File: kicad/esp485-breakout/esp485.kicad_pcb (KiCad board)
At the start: 2 copper layers, 25.4 x 26.2 mm, 15 parts, among them J1 Conn_01x08, J2 Conn_01x08, U1 MAX3485, U2 ESP-WROOM-02

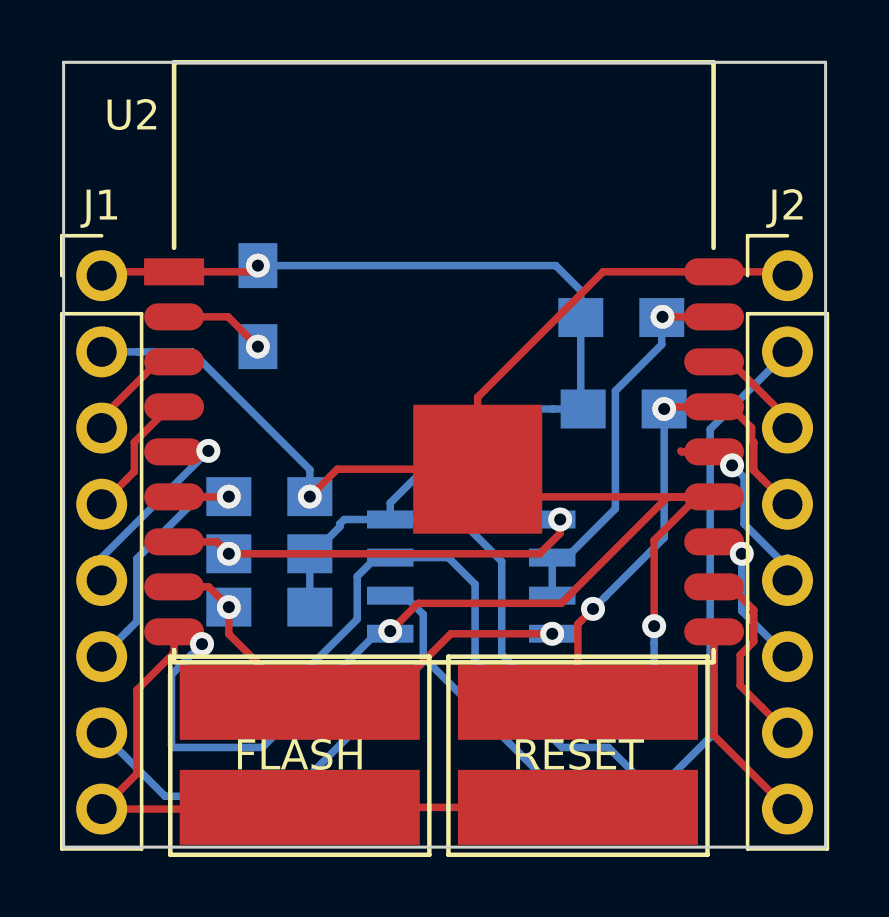
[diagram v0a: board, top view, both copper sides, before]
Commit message: all done probably
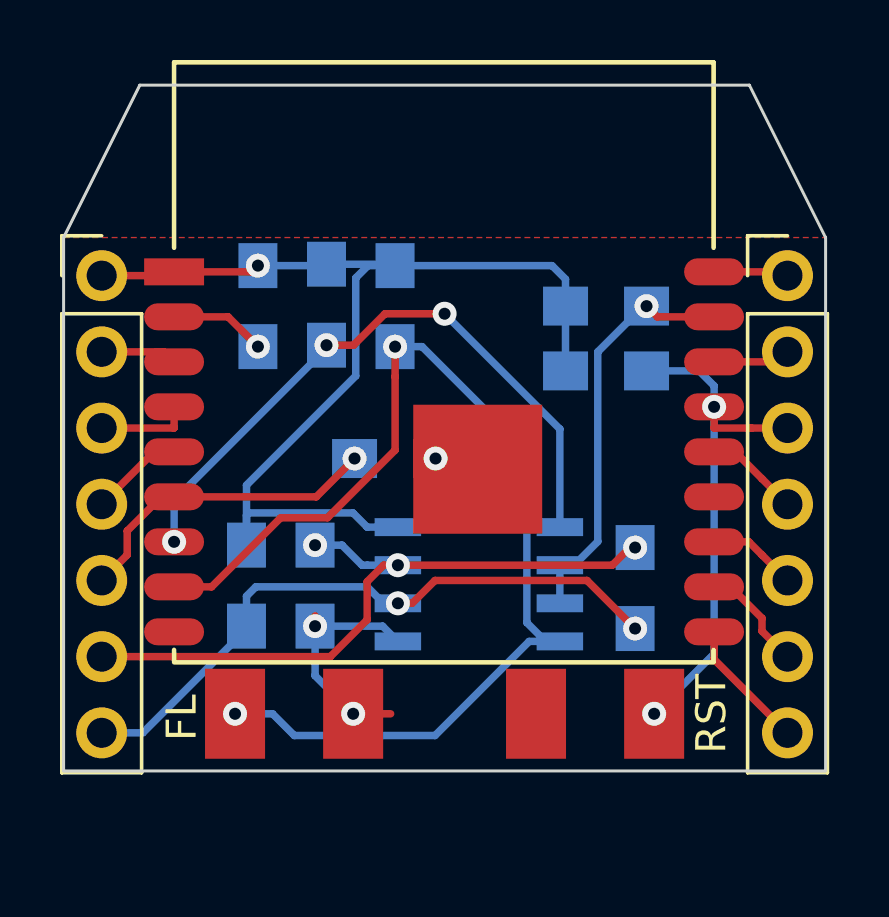
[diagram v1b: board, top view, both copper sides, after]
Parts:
- removed FLASH, RESET: SW_Push, tact:generic tactile switch
- added FL: SW_Push, tact:tactile_switch_smd_4x3mm_2p, F.Cu at (136.0, 111.1)
- added RST: SW_Push, tact:tactile_switch_smd_4x3mm_2p, F.Cu at (145.9, 111.1)
- J1, J2: value Conn_01x08 -> Conn_01x07; footprint Pin_Headers:Pin_Header_Straight_1x08_Pitch2.54mm -> Pin_Headers:Pin_Header_Straight_1x07_Pitch2.54mm
- moved R10 15.5 mm to (147.3, 106.9)
- moved R4 12.8 mm to (134.4, 106.9)
- moved R5 12.6 mm to (136.7, 106.9), turned to 270 degrees
- moved R3 10.9 mm to (139.3, 97.5), turned to 90 degrees
- moved R2 8.52 mm to (137.0, 97.5), turned to 90 degrees
- moved R9 4.38 mm to (139.3, 102.6)
- moved R7 1.40 mm to (146.4, 99.7)
- moved R8 0.64 mm to (146.4, 97.5)
- moved U1 0.36 mm to (142.1, 106.8)
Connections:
- J1 pad 2: GND -> Net-(J1-Pad2)
- R10 pad 1: Net-(J2-Pad2) -> Net-(J1-Pad6)
- R5 pad 1: Net-(J2-Pad2) -> Net-(J1-Pad6)
- R7 pad 2: Net-(J2-Pad4) -> Net-(J2-Pad3)
- R9 pad 1: Net-(J1-Pad6) -> Net-(J1-Pad5)
- U1 pad 7: Net-(J2-Pad2) -> Net-(J1-Pad6)
- U2 pad 10: Net-(J2-Pad8) -> Net-(J2-Pad7)
- U2 pad 11: Net-(J2-Pad7) -> Net-(J2-Pad6)
- U2 pad 12: Net-(J2-Pad6) -> Net-(J2-Pad5)
- U2 pad 14: Net-(J2-Pad5) -> Net-(J2-Pad4)
- U2 pad 15: Net-(J2-Pad4) -> Net-(J2-Pad3)
- U2 pad 16: Net-(J2-Pad3) -> Net-(J2-Pad2)
- U2 pad 3: Net-(J1-Pad3) -> Net-(J1-Pad2)
- U2 pad 4: Net-(J1-Pad4) -> Net-(J1-Pad3)
- U2 pad 5: Net-(J1-Pad5) -> Net-(J1-Pad4)
- U2 pad 6: Net-(J1-Pad6) -> Net-(J1-Pad5)
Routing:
- net GND: track 97.7 -> 11.0 mm, vias 4 -> 3
- net Net-(J2-Pad2): track 39.5 -> 2.58 mm
- net Net-(R3-Pad1): track 15.7 -> 38.0 mm
- net Net-(J2-Pad4): track 17.2 -> 3.17 mm, vias 2 -> 0
- net Net-(J2-Pad3): track 3.54 -> 17.4 mm, vias 0 -> 2
- net Net-(J1-Pad6): track 10.5 -> 23.1 mm, vias 1 -> 3
- net Net-(R2-Pad1): track 13.8 -> 21.6 mm, vias 2 -> 3
- net +3V3: track 44.9 -> 37.1 mm
- net Net-(J2-Pad8): track 6.92 -> 0.00 mm
- net Net-(J2-Pad5): track 7.27 -> 2.98 mm, vias 1 -> 0
- net Net-(J1-Pad5): track 6.95 -> 10.6 mm
- net Net-(J1-Pad7): track 23.8 -> 21.2 mm, vias 0 -> 2
- net Net-(J1-Pad2): track 0.00 -> 2.55 mm
- net Net-(J2-Pad7): track 6.58 -> 4.38 mm
- net Net-(R8-Pad2): track 12.8 -> 14.4 mm
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- added copper zone on F.Cu, net GND
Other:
- board size 25.4 x 26.2 mm -> 25.4 x 22.9 mm
- board text added: "3V3"
- board text added: "A"
- board text added: "B"
- board text added: "GND"
- board text added: "IO12"
- board text added: "IO13"
- board text added: "IO14"
- board text added: "IO15"
- board text added: "IO4"
- board text added: "IO5"
- board text added: "RST"
- board text added: "RXD"
- board text added: "TOUT"
- board text added: "TXD"
